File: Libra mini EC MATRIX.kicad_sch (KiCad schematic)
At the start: 72 parts, among them SW1 EC_SW, SW10 EC_SW, SW11 EC_SW, SW12 EC_SW, SW13 EC_SW, SW14 EC_SW, SW15 EC_SW, SW16 EC_SW, SW17 EC_SW, SW18 EC_SW, SW19 EC_SW, SW2 EC_SW, SW20 EC_SW, SW21 EC_SW, SW22 EC_SW, SW23 EC_SW, SW24 EC_SW, SW25 EC_SW, SW26 EC_SW, SW27 EC_SW, SW28 EC_SW, SW29 EC_SW, SW3 EC_SW, SW30 EC_SW, SW31 EC_SW, SW32 EC_SW, SW33 EC_SW, SW34 EC_SW, SW35 EC_SW, SW36 EC_SW, SW37 EC_SW, SW38 EC_SW, SW39 EC_SW, SW4 EC_SW, SW40 EC_SW, SW41 EC_SW, SW42 EC_SW, SW43 EC_SW, SW44 EC_SW, SW45 EC_SW, SW46 EC_SW, SW47 EC_SW, SW48 EC_SW, SW49 EC_SW, SW5 EC_SW, SW50 EC_SW, SW51 EC_SW, SW52 EC_SW, SW53 EC_SW, SW54 EC_SW, SW55 EC_SW, SW6 EC_SW, SW7 EC_SW, SW8 EC_SW, SW9 EC_SW

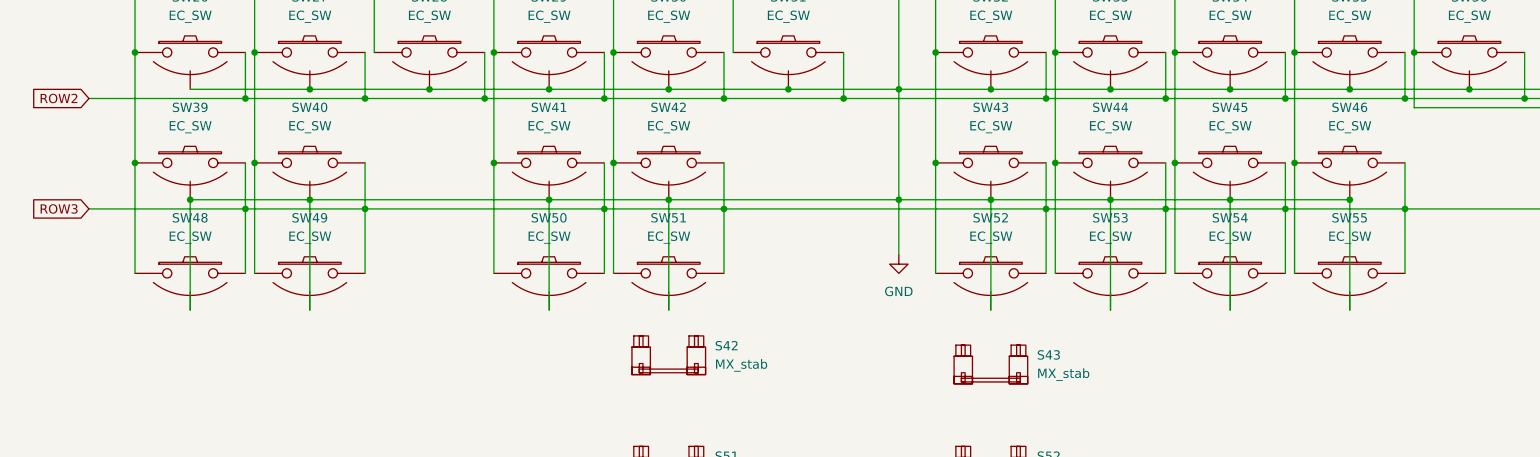
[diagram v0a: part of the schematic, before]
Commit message: 14.04.2026
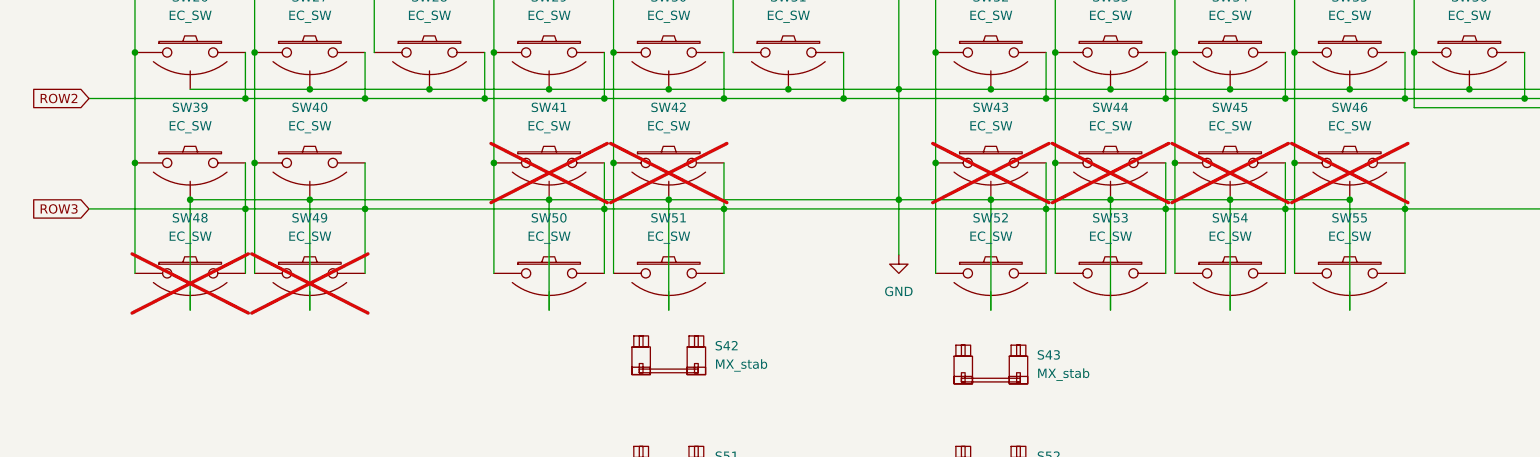
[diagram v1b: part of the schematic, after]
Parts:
- SW41, SW42, SW43, SW44, SW45, SW46, SW48, SW49: now not fitted; now left out of the parts list
- SW54, SW55: footprint Kicad footprints:ecs_pad_1U_hybrid_hotswap_V2 -> My_footprints:ecs_pad_hybrid_hotswap_1.25-1_libra_2.381
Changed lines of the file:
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@@
 		(unit 1)
 		(exclude_from_sim no)
-		(in_bom yes)
-		(on_board yes)
-		(dnp no)
+		(in_bom no)
+		(on_board no)
+		(dnp yes)
 		(fields_autoplaced yes)
 		(property "Reference" "SW46"
@@
 			)
 		)
-		(property "Footprint" "Kicad footprints:ecs_pad_1U_hybrid_hotswap_V2"
+		(property "Footprint" "My_footprints:ecs_pad_hybrid_hotswap_1.25-1_libra_2.381"
 			(at 201.93 102.87 0)
 			(effects
@@
 		(unit 1)
 		(exclude_from_sim no)
-		(in_bom yes)
-		(on_board yes)
-		(dnp no)
+		(in_bom no)
+		(on_board no)
+		(dnp yes)
 		(fields_autoplaced yes)
 		(property "Reference" "SW49"
@@
 		(unit 1)
 		(exclude_from_sim no)
-		(in_bom yes)
-		(on_board yes)
-		(dnp no)
+		(in_bom no)
+		(on_board no)
+		(dnp yes)
 		(fields_autoplaced yes)
 		(property "Reference" "SW42"
@@
 		(unit 1)
 		(exclude_from_sim no)
-		(in_bom yes)
-		(on_board yes)
-		(dnp no)
+		(in_bom no)
+		(on_board no)
+		(dnp yes)
 		(fields_autoplaced yes)
 		(property "Reference" "SW41"
@@
 		(unit 1)
 		(exclude_from_sim no)
-		(in_bom yes)
-		(on_board yes)
-		(dnp no)
+		(in_bom no)
+		(on_board no)
+		(dnp yes)
 		(fields_autoplaced yes)
 		(property "Reference" "SW43"
@@
 		(unit 1)
 		(exclude_from_sim no)
-		(in_bom yes)
-		(on_board yes)
-		(dnp no)
+		(in_bom no)
+		(on_board no)
+		(dnp yes)
 		(fields_autoplaced yes)
 		(property "Reference" "SW44"
@@
 		(unit 1)
 		(exclude_from_sim no)
-		(in_bom yes)
-		(on_board yes)
-		(dnp no)
+		(in_bom no)
+		(on_board no)
+		(dnp yes)
 		(fields_autoplaced yes)
 		(property "Reference" "SW45"
@@
 			)
 		)
-		(property "Footprint" "Kicad footprints:ecs_pad_1U_hybrid_hotswap_V2"
+		(property "Footprint" "My_footprints:ecs_pad_hybrid_hotswap_1.25-1_libra_2.381"
 			(at 185.42 102.87 0)
 			(effects
@@
 		(unit 1)
 		(exclude_from_sim no)
-		(in_bom yes)
-		(on_board yes)
-		(dnp no)
+		(in_bom no)
+		(on_board no)
+		(dnp yes)
 		(fields_autoplaced yes)
 		(property "Reference" "SW48"
